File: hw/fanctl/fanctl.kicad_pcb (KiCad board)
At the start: 2 copper layers, 76.2 x 27.9 mm, 28 parts, among them J1 FAN, J2 Screw_Terminal_01x06, M1 FAN, M2 FAN, M2.5 MountingHole_2.7mm_M2.5_ISO14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, Q1 BS170, Q2 BS170, Q3 BS170, Q4 BS170, U1 MCP9700-E

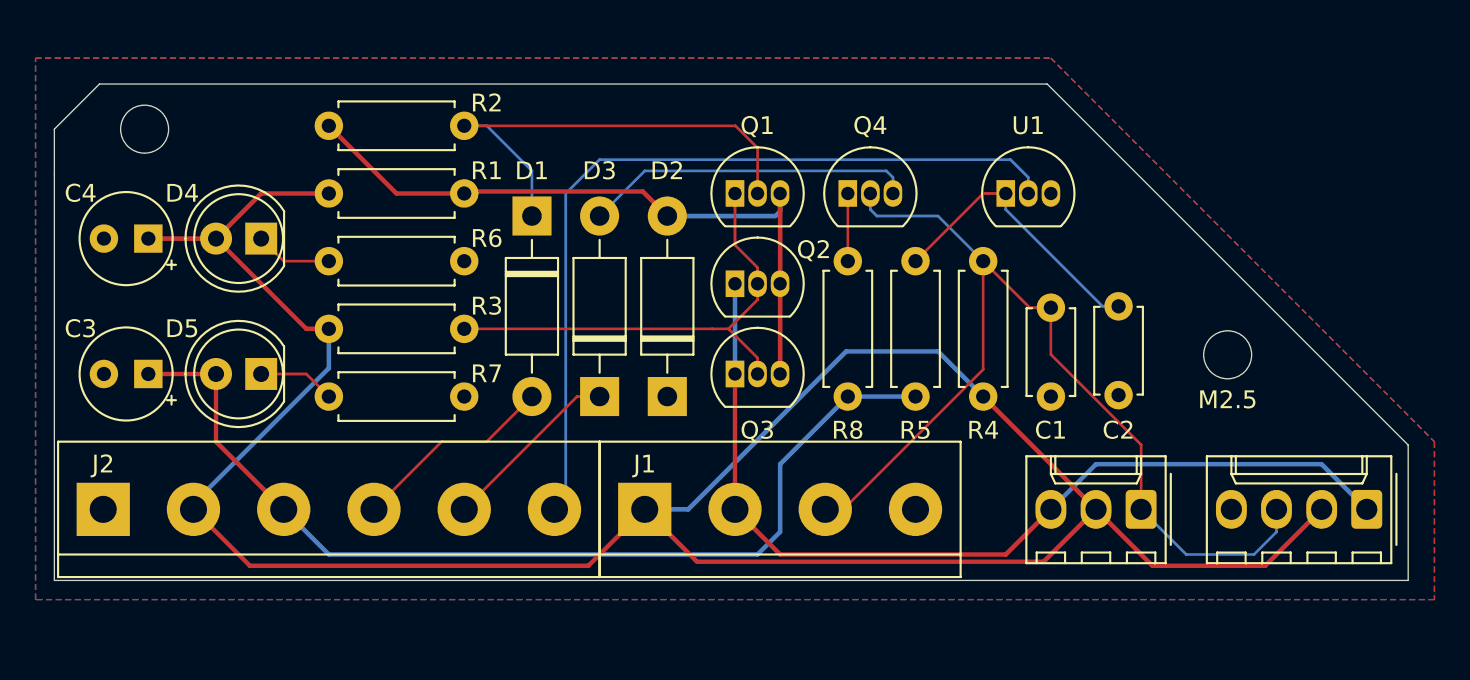
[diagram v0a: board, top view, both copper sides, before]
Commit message: layout done
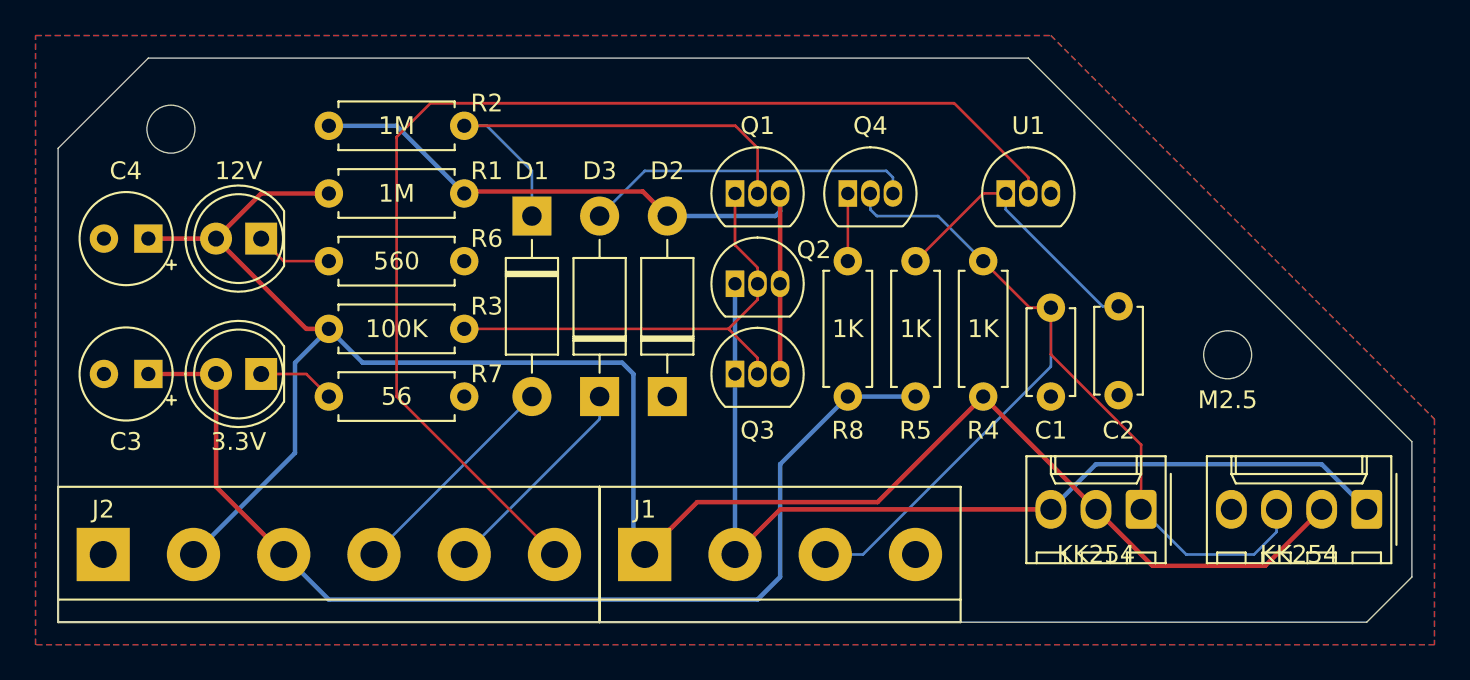
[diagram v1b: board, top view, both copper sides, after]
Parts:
- R5: value 0 -> 1K
- R6: value 470 -> 560
- R7: value 47 -> 56
- moved J1 2.54 mm to (132.1, 129.5)
- moved J2 2.54 mm to (101.6, 129.5)
- moved REF** 1.48 mm to (105.4, 105.6)
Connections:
- net Net-(J1-Pad2) renamed /FAN-
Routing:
- net +12V: track 136.9 -> 112.1 mm
- net /TEMP: track 46.3 -> 66.2 mm
- net +3V3: track 55.5 -> 60.6 mm
- net /TACI: track 55.5 -> 57.7 mm
- net /TACO: track 10.3 -> 12.0 mm
- net /FAN-: track 52.5 -> 54.0 mm
- net /PWM: track 11.5 -> 12.6 mm
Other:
- board size 76.2 x 27.9 mm -> 76.2 x 31.8 mm
- board text added: "+"
- board text added: "-"
- board text added: "100K"
- board text added: "1K"
- board text added: "1M"
- board text added: "3.3V"
- board text added: "56"
- board text added: "560"
- board text added: "KK254"
- board text added: "synack 2021 fanctl v1"
- board text removed: "FAN-"
